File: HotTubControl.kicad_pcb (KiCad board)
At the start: 2 copper layers, 90 x 90 mm, 33 parts, among them J1 Wasser Vorlauf, J2 Wasser Rücklauf, J3 Massagepumpe, J4 Filterpumpe, J5 Füllstandsensor, J6 Wagoklemme-4polig236-504_332-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, K1 JV-KT, K2 JV-KT, Q1 BC337, Q2 BSS138, Q3 BC337

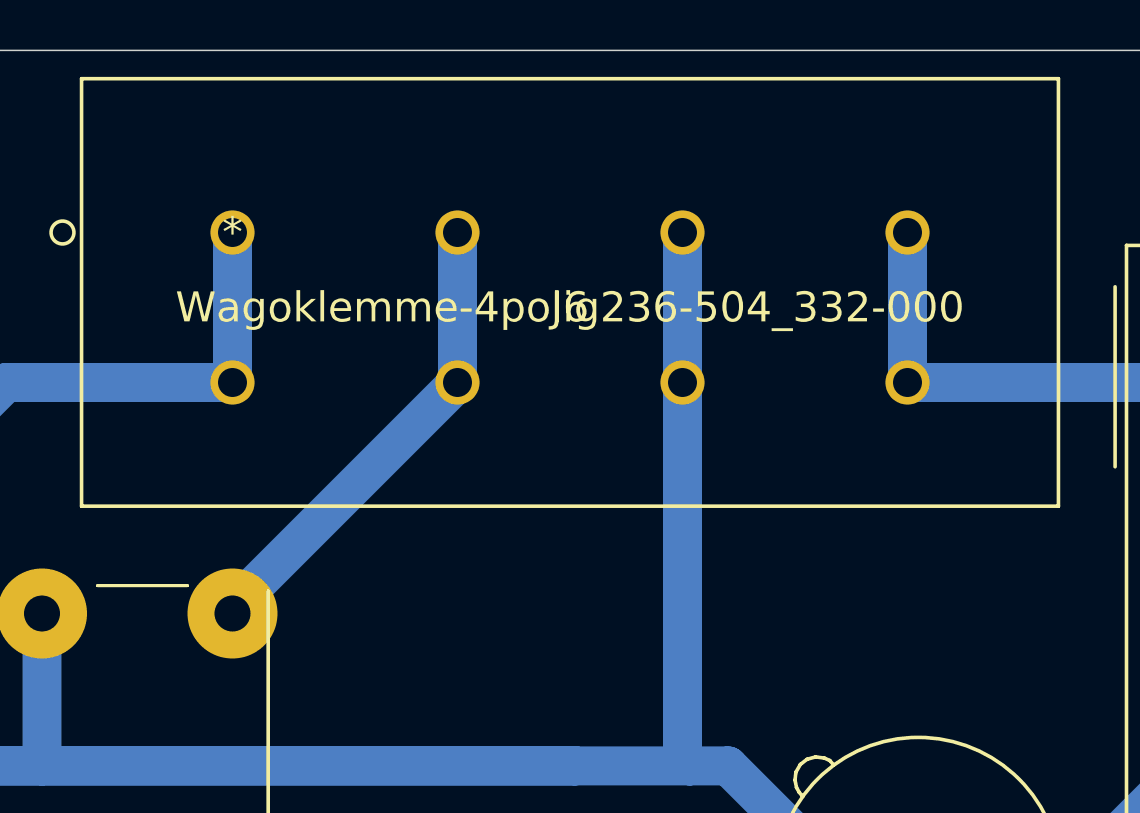
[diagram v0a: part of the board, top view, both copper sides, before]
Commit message: with ibom
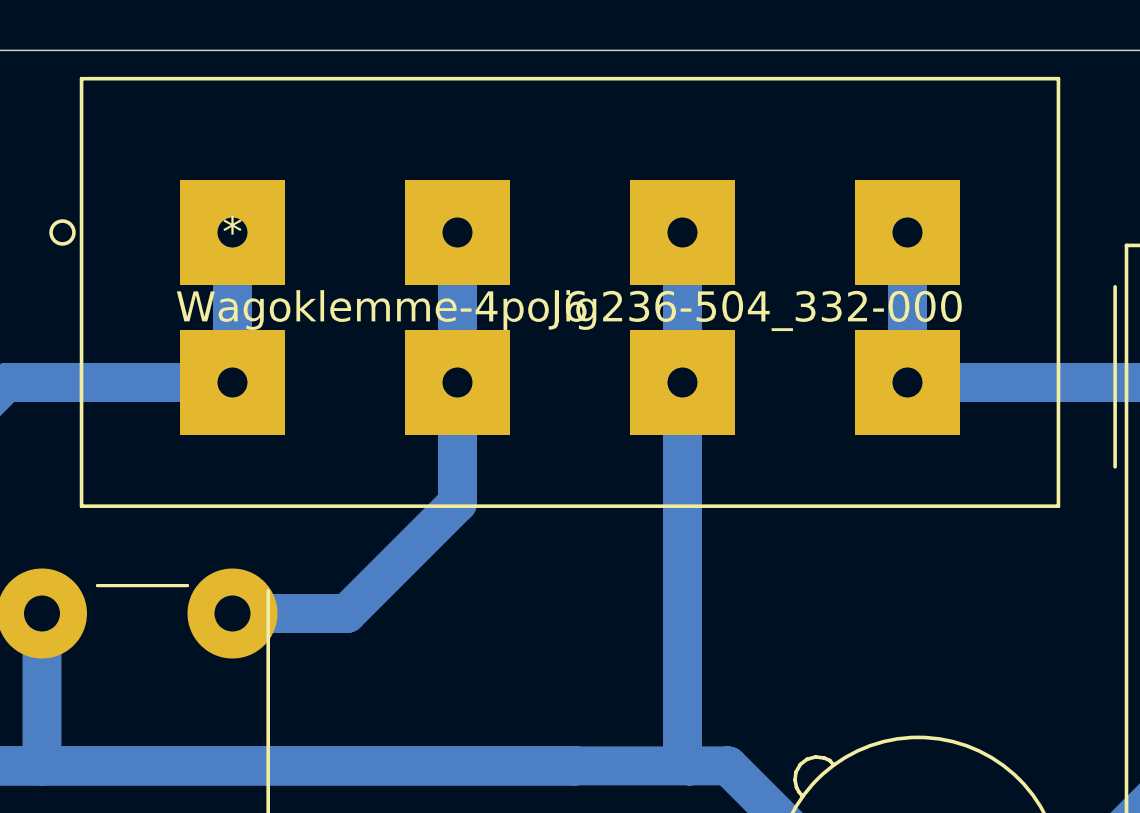
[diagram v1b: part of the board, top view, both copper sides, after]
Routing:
- net Net-(J6-Pad3): track 15.8 -> 18.0 mm
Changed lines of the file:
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@@
     (thickness 1.6)
     (drawings 8)
-    (tracks 246)
+    (tracks 247)
     (zones 0)
     (modules 33)
@@
     (add_net "Net-(Q2-Pad1)")
     (add_net "Net-(Q3-Pad2)")
+  )
+  (module ene9ba_footprint:WAGOKlemme4pol (layer F.Cu)
+    (at 79.25 63.42)
+    (fp_text reference J6 (at 11.25 2.5) (layer F.SilkS)
+      (effects (font (size 1 1) (thickness 0.15)))
+    )
+    (fp_text value Wagoklemme-4polig236-504_332-000 (at 11.25 2.5) (layer F.SilkS)
+      (effects (font (size 1 1) (thickness 0.15)))
+    )
+    (fp_line (start -5.0314 9.122415) (end 27.5314 9.122415) (layer F.SilkS) (width 0.12))
+    (fp_line (start 27.5314 9.122415) (end 27.5314 -5.126985) (layer F.SilkS) (width 0.12))
+    (fp_line (start 27.5314 -5.126985) (end -5.0314 -5.126985) (layer F.SilkS) (width 0.12))
+    (fp_line (start -5.0314 -5.126985) (end -5.0314 9.122415) (layer F.SilkS) (width 0.12))
+    (fp_line (start -4.9044 8.995415) (end 27.4044 8.995415) (layer F.Fab) (width 0.1))
+    (fp_line (start 27.4044 8.995415) (end 27.4044 -4.999985) (layer F.Fab) (width 0.1))
+    (fp_line (start 27.4044 -4.999985) (end -4.9044 -4.999985) (layer F.Fab) (width 0.1))
+    (fp_line (start -4.9044 -4.999985) (end -4.9044 8.995415) (layer F.Fab) (width 0.1))
+    (fp_line (start -5.1584 -5.253985) (end -5.1584 9.249415) (layer F.CrtYd) (width 0.05))
+    (fp_line (start -5.1584 9.249415) (end 27.6584 9.249415) (layer F.CrtYd) (width 0.05))
+    (fp_line (start 27.6584 9.249415) (end 27.6584 -5.253985) (layer F.CrtYd) (width 0.05))
+    (fp_line (start 27.6584 -5.253985) (end -5.1584 -5.253985) (layer F.CrtYd) (width 0.05))
+    (fp_circle (center 0 -1.905) (end 0.381 -1.905) (layer F.Fab) (width 0.1))
+    (fp_circle (center -5.6664 0) (end -5.2854 0) (layer F.SilkS) (width 0.12))
+    (fp_circle (center -5.6664 0) (end -5.2854 0) (layer B.SilkS) (width 0.12))
+    (fp_text user * (at 0 0) (layer F.Fab)
+      (effects (font (size 1 1) (thickness 0.15)))
+    )
+    (fp_text user * (at 0 0) (layer F.SilkS)
+      (effects (font (size 1 1) (thickness 0.15)))
+    )
+    (fp_text user "Copyright 2021 Accelerated Designs. All rights reserved." (at 0 0) (layer Cmts.User)
+      (effects (font (size 0.127 0.127) (thickness 0.002)))
+    )
+    (pad 8 thru_hole rect (at 22.5 5) (size 3.5 3.5) (drill 1) (layers *.Cu *.Mask)
+      (net 23 "Net-(J6-Pad7)"))
+    (pad 7 thru_hole rect (at 22.5 0) (size 3.5 3.5) (drill 1) (layers *.Cu *.Mask)
+      (net 23 "Net-(J6-Pad7)"))
+    (pad 6 thru_hole rect (at 15 5) (size 3.5 3.5) (drill 1) (layers *.Cu *.Mask)
+      (net 7 "Net-(F1-Pad2)"))
+    (pad 5 thru_hole rect (at 15 0) (size 3.5 3.5) (drill 1) (layers *.Cu *.Mask)
+      (net 7 "Net-(F1-Pad2)"))
+    (pad 4 thru_hole rect (at 7.5 5) (size 3.5 3.5) (drill 1) (layers *.Cu *.Mask)
+      (net 24 "Net-(J6-Pad3)"))
+    (pad 3 thru_hole rect (at 7.5 0) (size 3.5 3.5) (drill 1) (layers *.Cu *.Mask)
+      (net 24 "Net-(J6-Pad3)"))
+    (pad 2 thru_hole rect (at 0 5) (size 3.5 3.5) (drill 1) (layers *.Cu *.Mask)
+      (net 25 "Net-(J6-Pad1)"))
+    (pad 1 thru_hole rect (at 0 0) (size 3.5 3.5) (drill 1) (layers *.Cu *.Mask)
+      (net 25 "Net-(J6-Pad1)"))
+    (model ${KIPRJMOD}/3D-step/236-504_332-000.stp
+      (offset (xyz 28 0 0))
+      (scale (xyz 1 1 1))
+      (rotate (xyz -90 0 90))
+    )
   )
   (module Package_TO_SOT_THT:TO-92_Inline (layer F.Cu)
@@
     (model ${KIPRJMOD}/3D-step/IRM-03-5.stp
       (offset (xyz 8.5 -15 0))
-      (scale (xyz 1 1 1))
-      (rotate (xyz -90 0 90))
-    )
-  )
-  (module ene9ba_footprint:WAGOKlemme4pol (layer F.Cu)
-    (at 79.25 63.42)
-    (fp_text reference J6 (at 11.25 2.5) (layer F.SilkS)
-      (effects (font (size 1 1) (thickness 0.15)))
-    )
-    (fp_text value Wagoklemme-4polig236-504_332-000 (at 11.25 2.5) (layer F.SilkS)
-      (effects (font (size 1 1) (thickness 0.15)))
-    )
-    (fp_line (start -5.0314 9.122415) (end 27.5314 9.122415) (layer F.SilkS) (width 0.12))
-    (fp_line (start 27.5314 9.122415) (end 27.5314 -5.126985) (layer F.SilkS) (width 0.12))
-    (fp_line (start 27.5314 -5.126985) (end -5.0314 -5.126985) (layer F.SilkS) (width 0.12))
-    (fp_line (start -5.0314 -5.126985) (end -5.0314 9.122415) (layer F.SilkS) (width 0.12))
-    (fp_line (start -4.9044 8.995415) (end 27.4044 8.995415) (layer F.Fab) (width 0.1))
-    (fp_line (start 27.4044 8.995415) (end 27.4044 -4.999985) (layer F.Fab) (width 0.1))
-    (fp_line (start 27.4044 -4.999985) (end -4.9044 -4.999985) (layer F.Fab) (width 0.1))
-    (fp_line (start -4.9044 -4.999985) (end -4.9044 8.995415) (layer F.Fab) (width 0.1))
-    (fp_line (start -5.1584 -5.253985) (end -5.1584 9.249415) (layer F.CrtYd) (width 0.05))
-    (fp_line (start -5.1584 9.249415) (end 27.6584 9.249415) (layer F.CrtYd) (width 0.05))
-    (fp_line (start 27.6584 9.249415) (end 27.6584 -5.253985) (layer F.CrtYd) (width 0.05))
-    (fp_line (start 27.6584 -5.253985) (end -5.1584 -5.253985) (layer F.CrtYd) (width 0.05))
-    (fp_circle (center 0 -1.905) (end 0.381 -1.905) (layer F.Fab) (width 0.1))
-    (fp_circle (center -5.6664 0) (end -5.2854 0) (layer F.SilkS) (width 0.12))
-    (fp_circle (center -5.6664 0) (end -5.2854 0) (layer B.SilkS) (width 0.12))
-    (fp_text user * (at 0 0) (layer F.Fab)
-      (effects (font (size 1 1) (thickness 0.15)))
-    )
-    (fp_text user * (at 0 0) (layer F.SilkS)
-      (effects (font (size 1 1) (thickness 0.15)))
-    )
-    (fp_text user "Copyright 2021 Accelerated Designs. All rights reserved." (at 0 0) (layer Cmts.User)
-      (effects (font (size 0.127 0.127) (thickness 0.002)))
-    )
-    (pad 8 thru_hole circle (at 22.5 5) (size 1.4732 1.4732) (drill 0.9652) (layers *.Cu *.Mask)
-      (net 23 "Net-(J6-Pad7)"))
-    (pad 7 thru_hole circle (at 22.5 0) (size 1.4732 1.4732) (drill 0.9652) (layers *.Cu *.Mask)
-      (net 23 "Net-(J6-Pad7)"))
-    (pad 6 thru_hole circle (at 15 5) (size 1.4732 1.4732) (drill 0.9652) (layers *.Cu *.Mask)
-      (net 7 "Net-(F1-Pad2)"))
-    (pad 5 thru_hole circle (at 15 0) (size 1.4732 1.4732) (drill 0.9652) (layers *.Cu *.Mask)
-      (net 7 "Net-(F1-Pad2)"))
-    (pad 4 thru_hole circle (at 7.5 5) (size 1.4732 1.4732) (drill 0.9652) (layers *.Cu *.Mask)
-      (net 24 "Net-(J6-Pad3)"))
-    (pad 3 thru_hole circle (at 7.5 0) (size 1.4732 1.4732) (drill 0.9652) (layers *.Cu *.Mask)
-      (net 24 "Net-(J6-Pad3)"))
-    (pad 2 thru_hole circle (at 0 5) (size 1.4732 1.4732) (drill 0.9652) (layers *.Cu *.Mask)
-      (net 25 "Net-(J6-Pad1)"))
-    (pad 1 thru_hole circle (at 0 0) (size 1.4732 1.4732) (drill 0.9652) (layers *.Cu *.Mask)
-      (net 25 "Net-(J6-Pad1)"))
-    (model ${KIPRJMOD}/3D-step/236-504_332-000.stp
-      (offset (xyz 28 0 0))
       (scale (xyz 1 1 1))
       (rotate (xyz -90 0 90))
@@
   (segment (start 101.75 68.42) (end 111.09 68.42) (width 1.3) (layer B.Cu) (net 23))
   (segment (start 86.75 63.42) (end 86.75 68.42) (width 1.3) (layer B.Cu) (net 24))
-  (segment (start 79.25 75.92) (end 86.75 68.42) (width 1.3) (layer B.Cu) (net 24))
-  (segment (start 79.25 76.12) (end 79.25 75.92) (width 1.3) (layer B.Cu) (net 24))
+  (segment (start 86.75 72.43) (end 86.75 68.42) (width 1.3) (layer B.Cu) (net 24))
+  (segment (start 83.06 76.12) (end 86.75 72.43) (width 1.3) (layer B.Cu) (net 24))
+  (segment (start 79.25 76.12) (end 83.06 76.12) (width 1.3) (layer B.Cu) (net 24))
   (segment (start 79.25 68.42) (end 79.25 63.42) (width 1.3) (layer B.Cu) (net 25))
   (segment (start 71.71 68.42) (end 79.25 68.42) (width 1.3) (layer B.Cu) (net 25))
